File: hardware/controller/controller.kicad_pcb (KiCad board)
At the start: 2 copper layers, 100 x 69 mm, 210 parts, among them J1 USB_C_Receptacle_USB2.0_14P, J10 Conn_01x01, J11 Conn_01x01, J12 Conn_01x01, J13 Conn_02x03_Odd_Even, J2 IDC-10, J3 USB_C_Receptacle_USB2.0_14P, J4 XT-60, J5 Conn_01x07, J6 Conn_01x01, J7 Conn_01x01, J8 Conn_01x01, J9 Conn_02x03_Odd_Even, Q1 SUD50P04-08, Q10 AOD66406, Q11 AOD66406, Q12 AOD66406, Q13 AOD66406, Q2 AOD66406, Q3 AOD66406, Q4 AOD66406, Q5 AOD66406, Q6 AOD66406, Q7 AOD66406, Q8 AOD66406, Q9 AOD66406, SW1 SW_Push, SW2 SW_Push, SW3 SW_Push, SW4 SW_Push, SW5 SW_SPST, U1 USBLC6-2SC6, U10 LMV331, U11 IR2101, U12 LMV331, U13 IR2101, U14 LMV331, U15 IR2101, U16 LMV331, U17 IR2101, U18 LMV331, U19 IR2101, U2 ESP32-C3-WROOM-02, U20 LMV331, U3 STM32U535RET6, U5 USBLC6-2SC6, U6 LM1117MP-3.3, U7 LV14340, U8 MPU-6050, U9 IR2101, Y1 8MHz

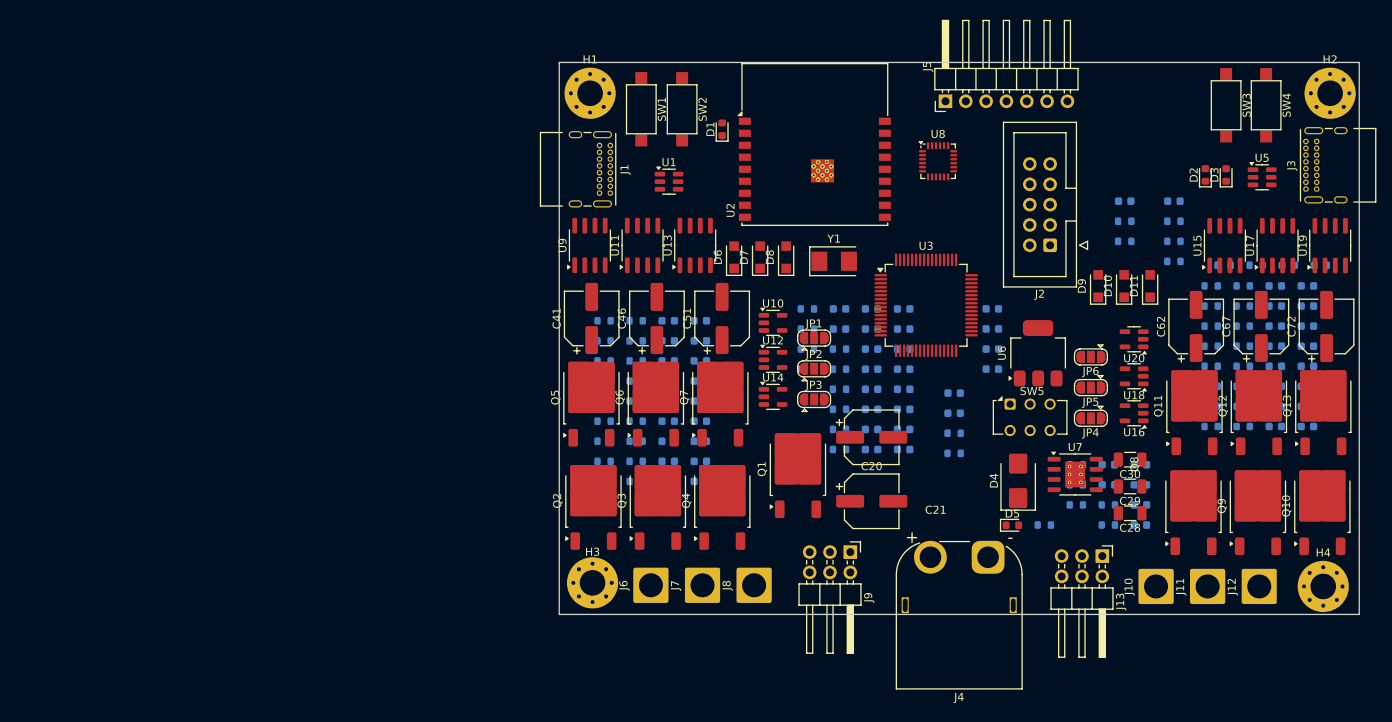
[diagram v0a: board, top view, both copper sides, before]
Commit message: custom footprints with all 3D models
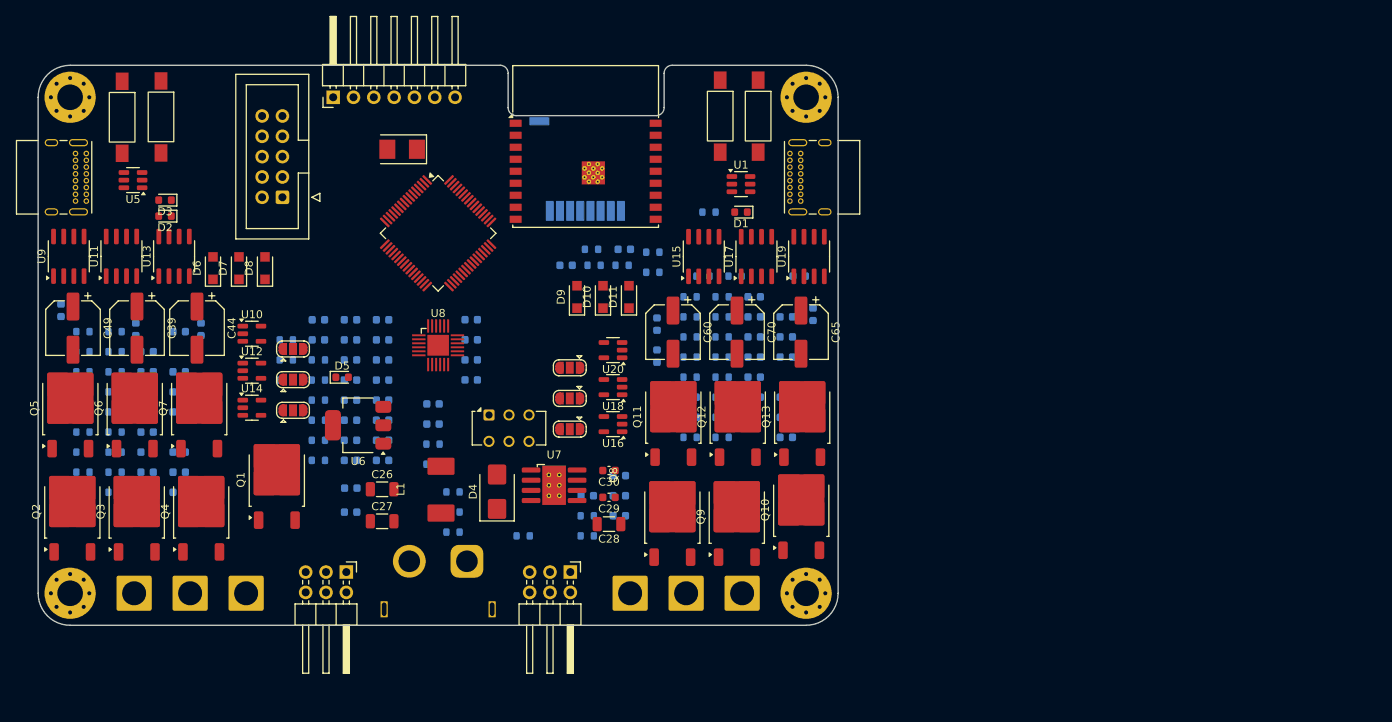
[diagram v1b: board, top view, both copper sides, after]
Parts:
- removed C78: 10u, Capacitor_SMD:C_0603_1608Metric
- removed C79: 100n, Capacitor_SMD:C_0603_1608Metric
- added L1: 6.8u/4.5A, hogger2:PA4341.XXXNLT, F.Cu at (150.4, 103.0)
- added U4: nRF24L01+ 2.4Gz Mini SMD, hogger2:nRF24L01p_Mini_SMD, B.Cu at (174.4, 68.5)
- C20, C51, C72: value 47u/50V -> 100n; footprint Capacitor_SMD:CP_Elec_6.3x7.7 -> Capacitor_SMD:C_0603_1608Metric; moved to B.Cu
- C21: value 47u/50V -> 100n/16V; footprint Capacitor_SMD:CP_Elec_6.3x7.7 -> Capacitor_SMD:C_0603_1608Metric; moved to B.Cu
- C23: value 100n/16V -> 4.7u
- C24: value 100n -> 4.7u
- C25: value 4.7u -> 100n
- C26: value 4.7u -> 10u/50V; footprint Capacitor_SMD:C_0603_1608Metric -> Capacitor_SMD:C_1206_3216Metric; moved to F.Cu
- C27: value 100n -> 47u/16V; footprint Capacitor_SMD:C_0603_1608Metric -> Capacitor_SMD:C_1206_3216Metric; moved to F.Cu
- C28: value 10u/50V -> 47u/16V
- C29: value 47u/16V -> 22n; footprint Capacitor_SMD:C_1206_3216Metric -> Capacitor_SMD:C_0603_1608Metric
- C30: value 47u/16V -> 100n; footprint Capacitor_SMD:C_1206_3216Metric -> Capacitor_SMD:C_0603_1608Metric
- C31: value 22n -> 100n
- C32, C53, C74: value 100n -> 10u
- C34, C56, C77: value 10u -> 100n
- C35: value 100n -> 2n2
- C36, C58: value 100n -> 1u/50V
- C37: value 2n2 -> 1u/50V
- C38, C43, C48, C59, C64, C69: value 1u/50V -> 100n
- C39, C44, C49, C60, C65, C70: value 1u/50V -> 47u/50V; footprint Capacitor_SMD:C_0603_1608Metric -> Capacitor_SMD:CP_Elec_6.3x7.7; moved to F.Cu
- C40, C45, C50, C61, C66, C71: value 100n -> 1n
- C41, C46, C62, C67: value 47u/50V -> 1u/50V; footprint Capacitor_SMD:CP_Elec_6.3x7.7 -> Capacitor_SMD:C_0603_1608Metric; moved to B.Cu
- C42, C47, C63, C68: value 1n -> 1u/50V
- C52, C73: value 1n -> 10u
- C57: value 10u -> 1u/50V
- J4: footprint Connector_AMASS:AMASS_XT60PW-M_1x02_P7.20mm_Horizontal -> hogger2:XT60PW-M
- SW1, SW2, SW3, SW4: footprint Button_Switch_SMD:SW_SPST_CK_RS282G05A3 -> hogger2:spst_6x3mm
- U7: footprint Package_SO:SOIC-8-1EP_3.9x4.9mm_P1.27mm_EP2.514x3.2mm_ThermalVias -> hogger2:LV14340
- U8: footprint Sensor_Motion:InvenSense_QFN-24_4x4mm_P0.5mm -> hogger2:MPU6050_handsolder
- moved J3 152.5 mm to (106.0, 61.0), turned to -90 degrees
- moved U5 141.1 mm to (111.9, 64.4), turned to 180 degrees
- moved SW4 138.1 mm to (115.4, 56.5)
- moved SW3 138.0 mm to (110.5, 56.5)
- moved D3 132.7 mm to (115.9, 66.9), turned to 180 degrees
- moved D2 130.2 mm to (115.9, 68.9), turned to 180 degrees
- moved J2 96.1 mm to (130.5, 66.5)
- moved C26 94.9 mm to (143.0, 103.0), turned to 0 degrees
- moved C27 91.1 mm to (143.0, 107.0), turned to 0 degrees
- moved D5 85.8 mm to (138.0, 89.0)
- moved U6 85.5 mm to (140.0, 95.0), turned to 180 degrees
- moved C60 79.5 mm to (179.4, 83.4), turned to -90 degrees
- moved R18 78.0 mm to (151.9, 103.3)
- moved R19 78.0 mm to (151.9, 105.8)
- moved R20 78.0 mm to (151.9, 108.4)
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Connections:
- C20 pad 1: /power/BATTERY_IN -> VBUS_SENSE
- C21 pad 1: VBUS -> Net-(U7-BOOT)
- C21 pad 2: GND -> Net-(D4-K)
- C22 pad 1: VBUS_SENSE -> +5V
- C23 pad 1: Net-(U7-BOOT) -> +5V
- C23 pad 2: Net-(D4-K) -> GND
- C24 pad 1: +5V -> +3.3V
- C25 pad 1: +5V -> +3.3V
- C26 pad 1: +3.3V -> VBUS
- C27 pad 1: +3.3V -> +5V
- C28 pad 1: VBUS -> +5V
- C29 pad 1: +5V -> Net-(U7-SS)
- C30 pad 1: +5V -> +3.3V
- C31 pad 1: Net-(U7-SS) -> +3.3V
- C34 pad 1: +3.3V -> /sensors/IMU_REGOUT
- C35 pad 1: +3.3V -> /sensors/IMU_CPOUT
- C36 pad 1: /sensors/IMU_REGOUT -> GND
- C36 pad 2: GND -> VBUS
- C37 pad 1: /sensors/IMU_CPOUT -> Net-(D6-K)
- C37 pad 2: GND -> /hog1/PHASE_U
- C38 pad 2: VBUS -> +3.3V
- C39 pad 1: Net-(D6-K) -> VBUS
- C39 pad 2: /hog1/PHASE_U -> GND
- C40 pad 1: GND -> /hog1/BEMF_U
- C40 pad 2: +3.3V -> GND
- C41 pad 1: VBUS -> GND
- C41 pad 2: GND -> VBUS
- C42 pad 1: /hog1/BEMF_U -> Net-(D7-K)
- C42 pad 2: GND -> /hog1/PHASE_V
- C43 pad 2: VBUS -> +3.3V
- C44 pad 1: Net-(D7-K) -> VBUS
- C44 pad 2: /hog1/PHASE_V -> GND
- C45 pad 1: GND -> /hog1/BEMF_V
- C45 pad 2: +3.3V -> GND
- C46 pad 1: VBUS -> GND
- C46 pad 2: GND -> VBUS
- C47 pad 1: /hog1/BEMF_V -> Net-(D8-K)
- C47 pad 2: GND -> /hog1/PHASE_W
- C48 pad 2: VBUS -> +3.3V
- C49 pad 1: Net-(D8-K) -> VBUS
- C49 pad 2: /hog1/PHASE_W -> GND
- C50 pad 1: GND -> /hog1/BEMF_W
- C50 pad 2: +3.3V -> GND
- C51 pad 1: VBUS -> +5V
- C52 pad 1: /hog1/BEMF_W -> +5V
- C57 pad 1: +5V -> GND
- C57 pad 2: GND -> VBUS
- C58 pad 1: +5V -> Net-(D9-K)
- C58 pad 2: GND -> /hog2/PHASE_U
- C59 pad 2: VBUS -> +3.3V
- C60 pad 1: Net-(D9-K) -> VBUS
- C60 pad 2: /hog2/PHASE_U -> GND
- C61 pad 1: GND -> /hog2/BEMF_U
- C61 pad 2: +3.3V -> GND
- C62 pad 1: VBUS -> GND
- C62 pad 2: GND -> VBUS
- C63 pad 1: /hog2/BEMF_U -> Net-(D10-K)
- C63 pad 2: GND -> /hog2/PHASE_V
- C64 pad 2: VBUS -> +3.3V
- C65 pad 1: Net-(D10-K) -> VBUS
- C65 pad 2: /hog2/PHASE_V -> GND
- C66 pad 1: GND -> /hog2/BEMF_V
- C66 pad 2: +3.3V -> GND
- C67 pad 1: VBUS -> GND
- C67 pad 2: GND -> VBUS
- C68 pad 1: /hog2/BEMF_V -> Net-(D11-K)
- C68 pad 2: GND -> /hog2/PHASE_W
- C69 pad 2: VBUS -> +3.3V
- C70 pad 1: Net-(D11-K) -> VBUS
- C70 pad 2: /hog2/PHASE_W -> GND
- C71 pad 1: GND -> /hog2/BEMF_W
- C71 pad 2: +3.3V -> GND
- C72 pad 1: VBUS -> +5V
- C73 pad 1: /hog2/BEMF_W -> +5V
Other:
- board size 100 x 69 mm -> 100 x 70 mm
